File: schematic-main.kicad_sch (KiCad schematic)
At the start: 11 parts, among them J1 Battery converter, J2 CAN, J3 FUEL CELL, J4 Joulemeter, J5 MOTOR CONTROLER, J6 SUPER CAPACITORS, P1 USB_C_Plug_USB2.0

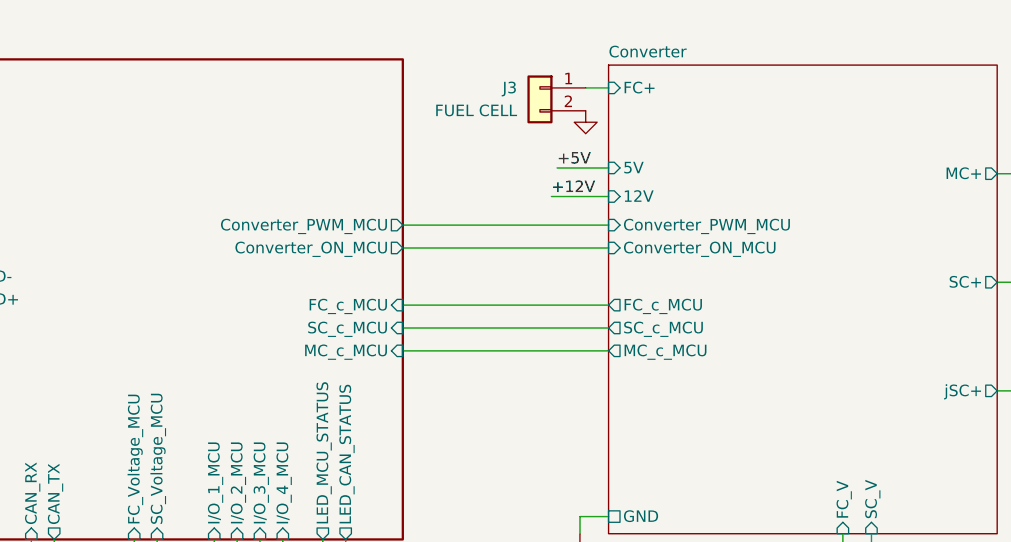
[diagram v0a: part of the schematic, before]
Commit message: Buck - boost converter
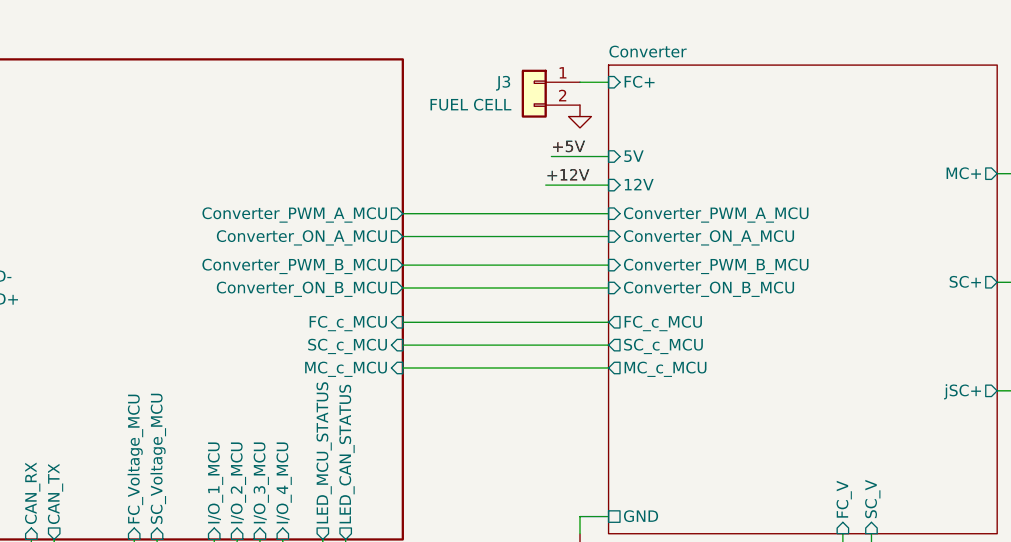
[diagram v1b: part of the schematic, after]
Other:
- sheet Converter ports: added Converter_ON_A_MCU, Converter_ON_B_MCU, Converter_PWM_A_MCU, Converter_PWM_B_MCU; removed Converter_ON_MCU, Converter_PWM_MCU
- sheet MCU ports: added Converter_ON_A_MCU, Converter_ON_B_MCU, Converter_PWM_A_MCU, Converter_PWM_B_MCU; removed Converter_ON_MCU, Converter_PWM_MCU
- moved on the sheet: J3
